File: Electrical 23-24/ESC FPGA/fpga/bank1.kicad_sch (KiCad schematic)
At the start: 2 parts, among them U1 XC6SLX4-TQG144

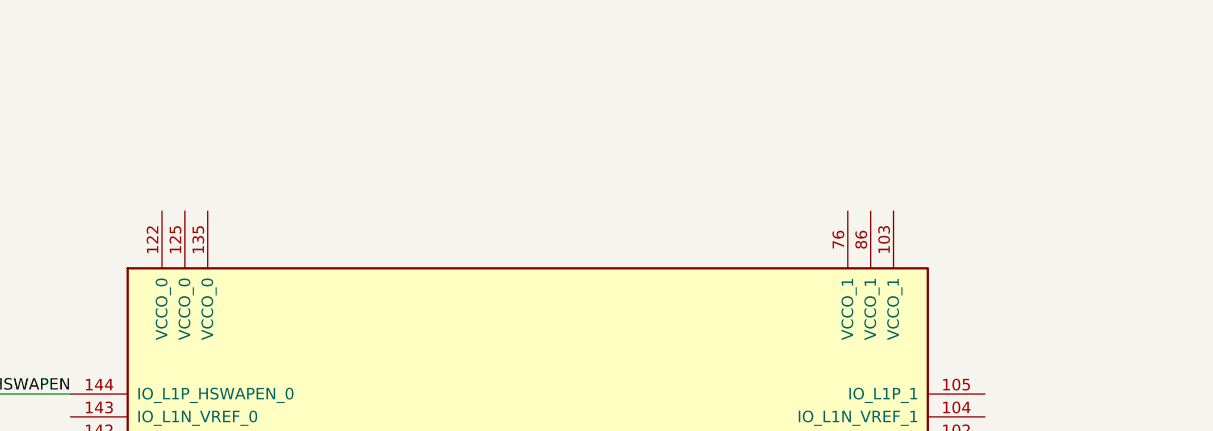
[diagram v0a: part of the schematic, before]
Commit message: idk but something
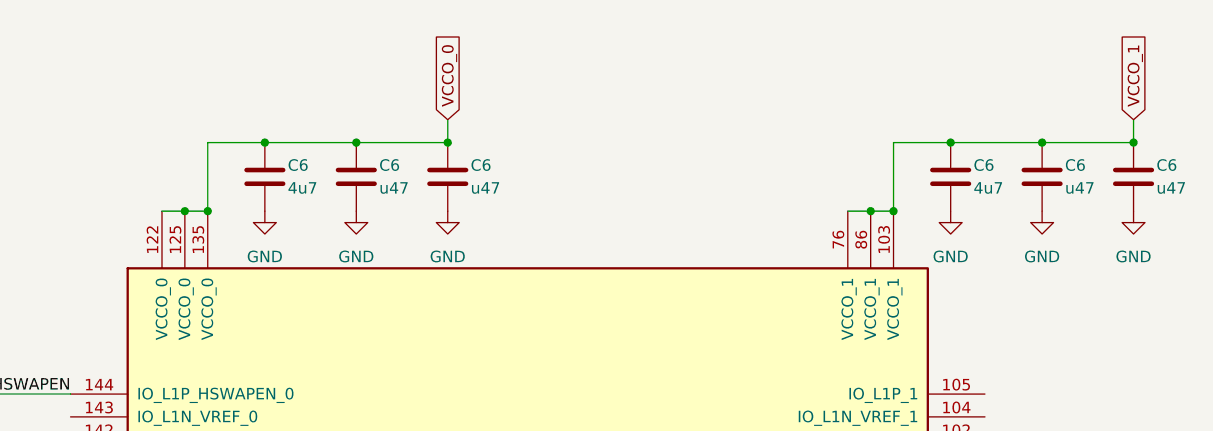
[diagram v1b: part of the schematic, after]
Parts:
- added C6 (x2): 4u7, symbol Device:C
- added C6 (x4): u47, symbol Device:C
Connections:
- net GND: now also C6.2, C6.2, C6.2, C6.2, C6.2, C6.2
- net VCCO_1: now reaches U1.103 (VCCO_1)
- net VCCO_1: now also U1.76 (VCCO_1), U1.86 (VCCO_1), C6.1, C6.1, C6.1
- net VCCO_0: now reaches U1.122 (VCCO_0)
- net VCCO_0: now also U1.125 (VCCO_0), U1.135 (VCCO_0), C6.1, C6.1, C6.1
